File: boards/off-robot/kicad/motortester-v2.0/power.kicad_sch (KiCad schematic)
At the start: 5 parts, among them U301 VND5E006ASPTR-E, U302 MPM3620GQV-P, U303 MPM3620GQV-P, U304 MPM3620GQV-P, U305 MPM3620GQV-P

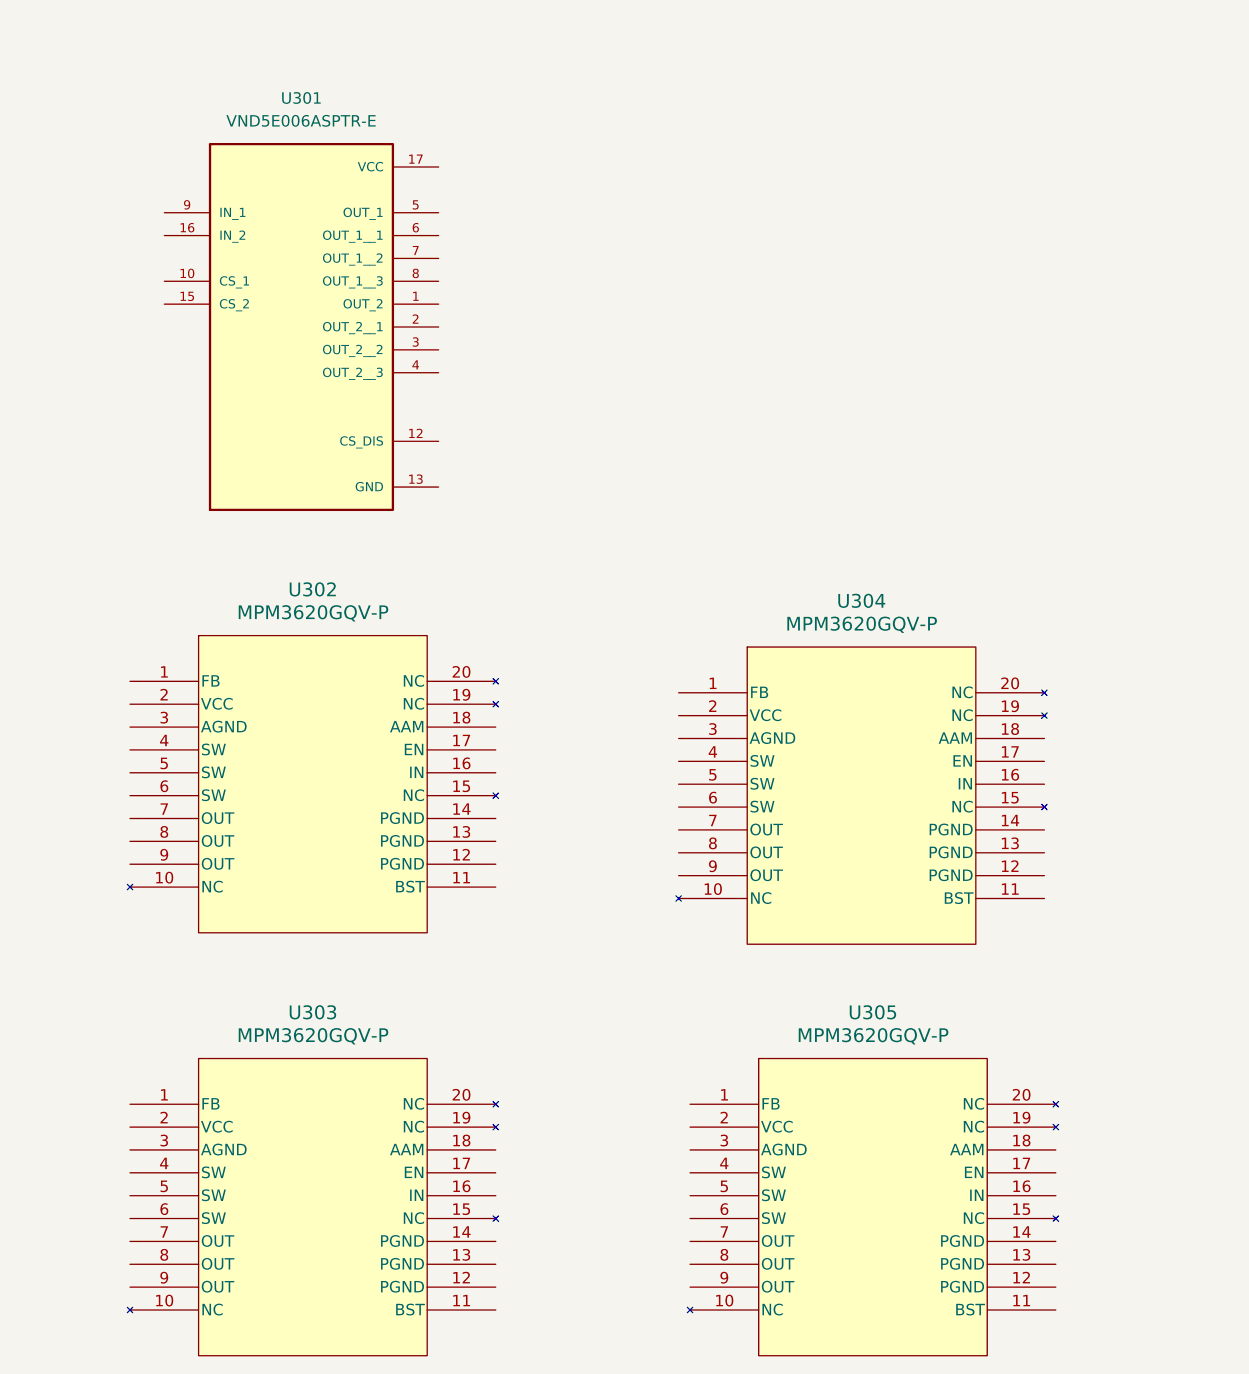
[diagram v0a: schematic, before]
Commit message: finished new motor driver poc
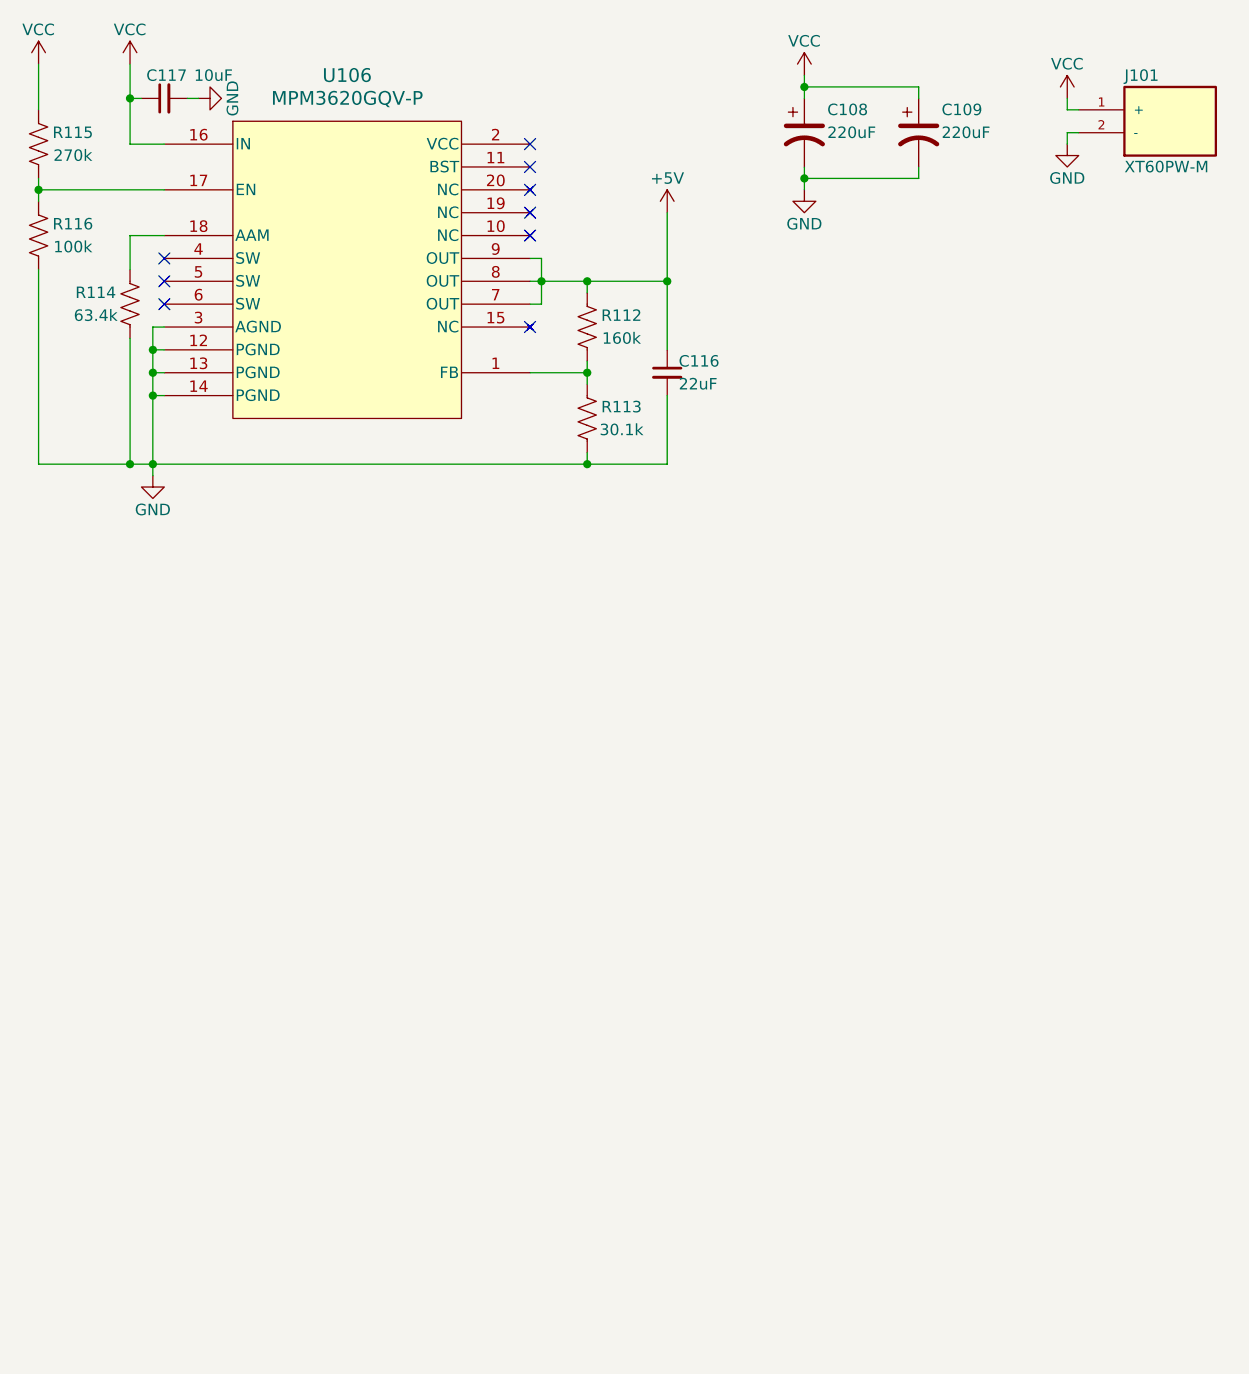
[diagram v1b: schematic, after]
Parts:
- removed U301: VND5E006ASPTR-E, lib:IC_VND5E006ASPTR-E, symbol lib:VND5E006ASPTR-E
- removed U302, U303, U304, U305: MPM3620GQV-P, lib:MPM3620GQV-P, symbol lib:MPM3620GQV-P
- added C108, C109: 220uF, Capacitor_THT:CP_Radial_D10.0mm_P5.00mm, symbol Device:C_Polarized_US
- added C116: 22uF, Resistor_SMD:R_1206_3216Metric, symbol Device:C_Small
- added C117: 10uF, Resistor_SMD:R_1206_3216Metric, symbol Device:C_Small
- added J101: XT60PW-M, lib:AMASS_XT60PW-M, symbol lib:XT60PW-M
- added R112: 160k, Resistor_SMD:R_0603_1608Metric, symbol Device:R_US
- added R113: 30.1k, Resistor_SMD:R_0603_1608Metric, symbol Device:R_US
- added R114: 63.4k, Resistor_SMD:R_0603_1608Metric, symbol Device:R_US
- added R115: 270k, Resistor_SMD:R_0603_1608Metric, symbol Device:R_US
- added R116: 100k, Resistor_SMD:R_0603_1608Metric, symbol Device:R_US
- added U106: MPM3620GQV-P, lib:MPM3620GQV-P, symbol lib:MPM3620GQV-P
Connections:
- new net: R112.1, R113.2, U106.1 (FB)
- new net: R115.1, R116.2, U106.17 (EN)
- new net: R114.2, U106.18 (AAM)
- new net +5V: C116.1, R112.2, U106.7 (OUT), U106.8 (OUT), U106.9 (OUT)
- new net GND: C108.2, C109.2, C116.2, C117.2, J101.2 (-), R113.1, R114.1, R116.1, U106.12 (PGND), U106.13 (PGND), U106.14 (PGND), U106.3 (AGND)
- new net VCC: C108.1, C109.1, C117.1, J101.1 (+), R115.2, U106.16 (IN)
- no-connect marks 0 -> 9
